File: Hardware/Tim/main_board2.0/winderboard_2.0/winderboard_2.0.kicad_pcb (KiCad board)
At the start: 4 copper layers, 63.8 x 113 mm, 59 parts, among them J1 Temp Probe 1, J10 XBee Explorer, J11 BNO055, J12 IR Temp Sensor, J13 Conn_01x02_Socket, J14 Conn_Coaxial, J15 I2C Pinout, J16 INA260, J17 Conn_01x04_Socket, J18 Conn_01x08_Pin, J19 Conn_01x01_Pin, J2 Temp Probe 2, J3 Limit Switch 2, J4 Limit Switch 1, J5 Encoder 1, J6 Encoder 2, J7 ESC, J8 Heater 1, J9 Heater 2, M1 Stepper_Motor_bipolar, M2 Motor_Servo, Q1 NMOS, Q2 NMOS, Q3 DMN6040SK3-13, U1 DEV-16771, U2 MS5607-02BA, U3 MAX-M10S, U5 LM1084-ADJ, U6 0.3 Ohm Resistor, U8 TPS62133

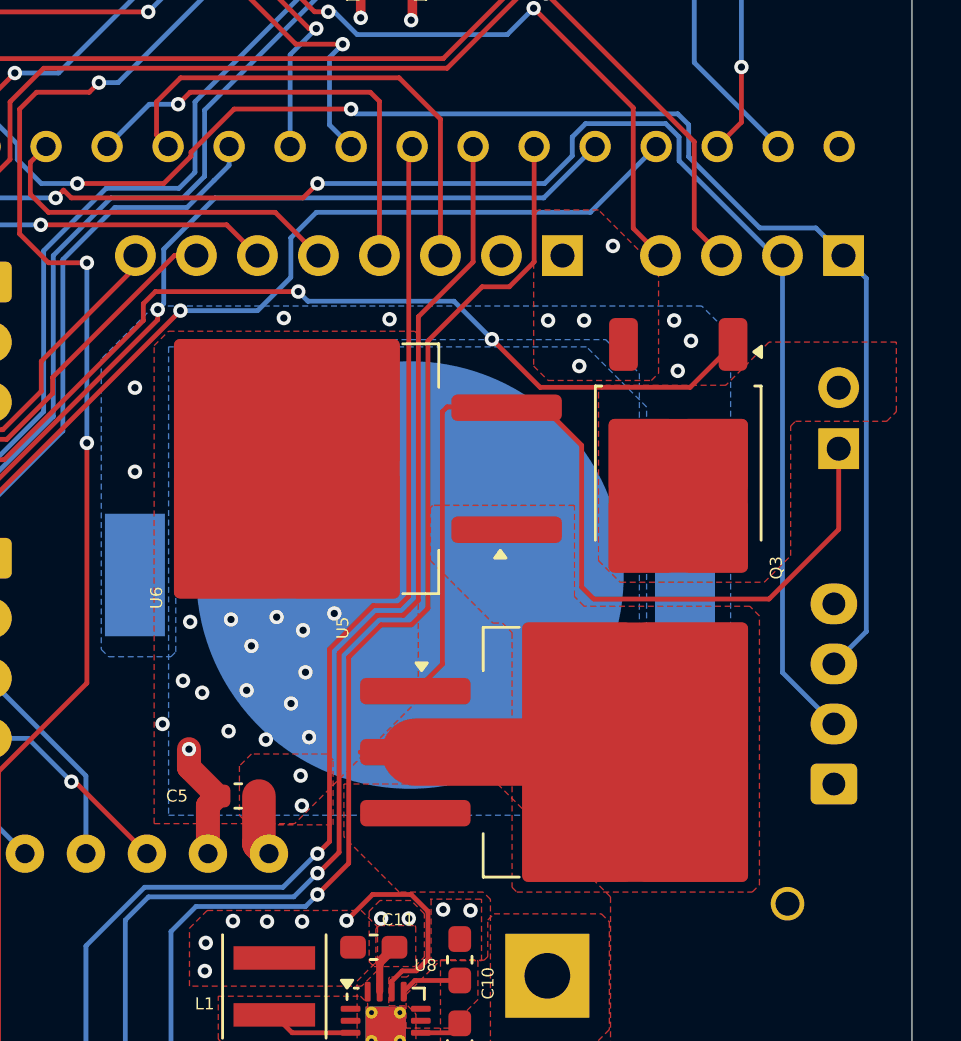
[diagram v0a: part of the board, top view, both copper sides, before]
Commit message: recovered from covid push
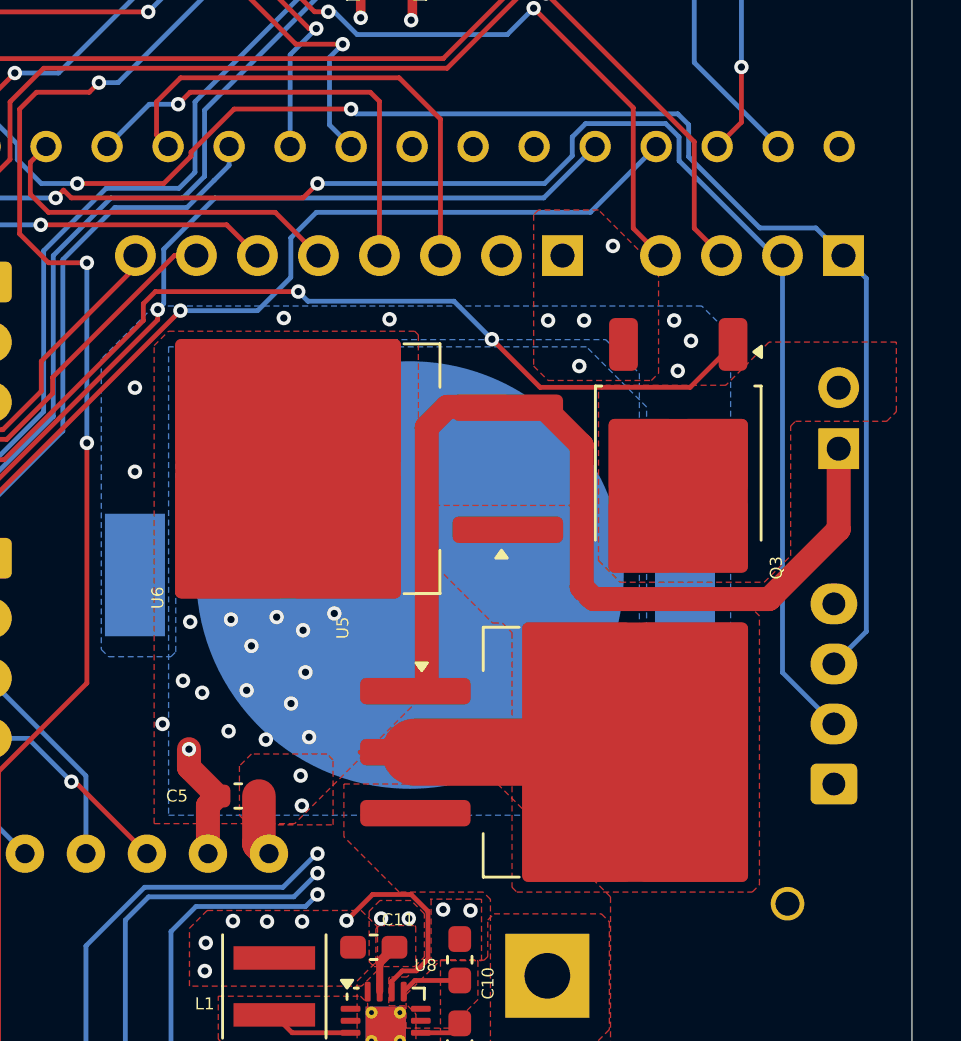
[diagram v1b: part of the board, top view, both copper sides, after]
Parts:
- moved U6 0.05 mm to (198.3, 117.1)
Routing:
- net stepper_MS1: track 53.1 -> 51.7 mm
- net stepper_MS2: track 52.7 -> 52.1 mm
- net stepper_MS3: track 51.8 -> 51.2 mm
